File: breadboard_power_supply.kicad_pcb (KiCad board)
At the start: 2 copper layers, 46.7 x 52.3 mm, 18 parts, among them J1 Barrel_Jack_Switch, J2 locked, J3 Conn_01x02_Male, J4 Screw_Terminal_01x02, J5 Conn_01x03_Male, J6 Conn_01x03_Male, J7 Screw_Terminal_01x02, U1 LM7805_TO220, U2 LM317_TO-220

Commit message: PCB complete design of the power supply.
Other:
- board text added: "0,2000 mm / 0,0000 mm"
- board text added: "0,3000 mm"
- board text added: "1,6000 mm"
- board text added: "2"
- board text added: "46,8360 mm x 52,4240 mm"
- board text added: "BOARD CHARACTERISTICS"
- board text added: "Board Thickness:"
- board text added: "Board overall dimensions:"
- board text added: "Castellated pads:"
- board text added: "Copper Finish:"
- board text added: "Copper Layer Count:"
- board text added: "Edge card connectors:"
- board text added: "Impedance Control:"
- board text added: "Min hole diameter:"
- board text added: "Min track/spacing:"
- board text added: "No"
- board text added: "None"
- board text added: "Plated Board Edge:"
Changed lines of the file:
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@@
     (effects (font (size 0.8 0.8) (thickness 0.1)))
+  )
+  (gr_text "Castellated pads: " (at 60.694 77.316) (layer "User.1")
+    (effects (font (size 1.5 1.5) (thickness 0.2)) (justify left top))
+  )
+  (gr_text "Min hole diameter: " (at 127.308286 68.286) (layer "User.1")
+    (effects (font (size 1.5 1.5) (thickness 0.2)) (justify left top))
+  )
+  (gr_text "No" (at 152.151143 77.316) (layer "User.1")
+    (effects (font (size 1.5 1.5) (thickness 0.2)) (justify left top))
+  )
+  (gr_text "Copper Layer Count: " (at 60.694 59.256) (layer "User.1")
+    (effects (font (size 1.5 1.5) (thickness 0.2)) (justify left top))
+  )
+  (gr_text "No" (at 93.251143 81.831) (layer "User.1")
+    (effects (font (size 1.5 1.5) (thickness 0.2)) (justify left top))
+  )
+  (gr_text "" (at 127.308286 63.771) (layer "User.1")
+    (effects (font (size 1.5 1.5) (thickness 0.2)) (justify left top))
+  )
+  (gr_text "No" (at 93.251143 77.316) (layer "User.1")
+    (effects (font (size 1.5 1.5) (thickness 0.2)) (justify left top))
+  )
+  (gr_text "Board overall dimensions: " (at 60.694 63.771) (layer "User.1")
+    (effects (font (size 1.5 1.5) (thickness 0.2)) (justify left top))
+  )
+  (gr_text "Copper Finish: " (at 60.694 72.801) (layer "User.1")
+    (effects (font (size 1.5 1.5) (thickness 0.2)) (justify left top))
+  )
+  (gr_text "Edge card connectors: " (at 60.694 81.831) (layer "User.1")
+    (effects (font (size 1.5 1.5) (thickness 0.2)) (justify left top))
+  )
+  (gr_text "2" (at 93.251143 59.256) (layer "User.1")
+    (effects (font (size 1.5 1.5) (thickness 0.2)) (justify left top))
+  )
+  (gr_text "No" (at 152.151143 72.801) (layer "User.1")
+    (effects (font (size 1.5 1.5) (thickness 0.2)) (justify left top))
+  )
+  (gr_text "1,6000 mm" (at 152.151143 59.256) (layer "User.1")
+    (effects (font (size 1.5 1.5) (thickness 0.2)) (justify left top))
+  )
+  (gr_text "Board Thickness: " (at 127.308286 59.256) (layer "User.1")
+    (effects (font (size 1.5 1.5) (thickness 0.2)) (justify left top))
+  )
+  (gr_text "None" (at 93.251143 72.801) (layer "User.1")
+    (effects (font (size 1.5 1.5) (thickness 0.2)) (justify left top))
+  )
+  (gr_text "Min track/spacing: " (at 60.694 68.286) (layer "User.1")
+    (effects (font (size 1.5 1.5) (thickness 0.2)) (justify left top))
+  )
+  (gr_text "0,2000 mm / 0,0000 mm" (at 93.251143 68.286) (layer "User.1")
+    (effects (font (size 1.5 1.5) (thickness 0.2)) (justify left top))
+  )
+  (gr_text "BOARD CHARACTERISTICS" (at 59.944 53.086) (layer "User.1")
+    (effects (font (size 2 2) (thickness 0.4)) (justify left top))
+  )
+  (gr_text "" (at 152.151143 63.771) (layer "User.1")
+    (effects (font (size 1.5 1.5) (thickness 0.2)) (justify left top))
+  )
+  (gr_text "Impedance Control: " (at 127.308286 72.801) (layer "User.1")
+    (effects (font (size 1.5 1.5) (thickness 0.2)) (justify left top))
+  )
+  (gr_text "0,3000 mm" (at 152.151143 68.286) (layer "User.1")
+    (effects (font (size 1.5 1.5) (thickness 0.2)) (justify left top))
+  )
+  (gr_text "Plated Board Edge: " (at 127.308286 77.316) (layer "User.1")
+    (effects (font (size 1.5 1.5) (thickness 0.2)) (justify left top))
+  )
+  (gr_text "46,8360 mm x 52,4240 mm" (at 93.251143 63.771) (layer "User.1")
+    (effects (font (size 1.5 1.5) (thickness 0.2)) (justify left top))
   )
   (dimension (type aligned) (layer "User.1")
@@
     )
   )
+  (group "group-boardCharacteristics" (id 3579cf2f-29b0-46b6-a07d-483fb5586322)
+    (members
+      044dde97-ee2e-473a-9264-ed4dff1893a5
+      15ea3484-2685-47cb-9e01-ec01c6d477b8
+      18d3014d-7089-41b5-ab03-53cc0a265580
+      232ccf4f-3322-4e62-990b-290e6ff36fcd
+      3f96e159-1f3b-4ee7-a46e-e60d78f2137a
+      406d491e-5b01-46dc-a768-fd0992cdb346
+      4160bbf7-ffff-4c5c-a647-5ee58ddecf06
+      42b61d5b-39d6-462b-b2cc-57656078085f
+      661ca2ba-bce5-4308-99a6-de333a625515
+      662bafcb-dcfb-4471-a8a9-f5c777fdf249
+      6d7ff8c0-8a2a-4636-844f-c7210ff3e6f2
+      720ec55a-7c69-4064-b792-ef3dbba4eab9
+      722636b6-8ff0-452f-9357-23deb317d921
+      7582a530-a952-46c1-b7eb-75006524ba29
+      8ae05d37-86b4-45ea-800f-f1f9fb167857
+      93ac15d8-5f91-4361-acff-be4992b93b51
+      96781640-c07e-4eea-a372-067ded96b703
+      bf8d857b-70bf-41ee-a068-5771461e04e9
+      c6462399-f2e4-4f1a-b34a-b49a04c8bdb9
+      d115a0df-1034-4583-83af-ff1cb8acfa17
+      d4ef5db0-5fba-4fcd-ab64-2ef2646c5c6d
+      e000728f-e3c5-4fc4-86af-db9ceb3a6542
+      f284b1e2-75a4-4a3f-a5f4-6f05f15fb4f5
+    )
+  )

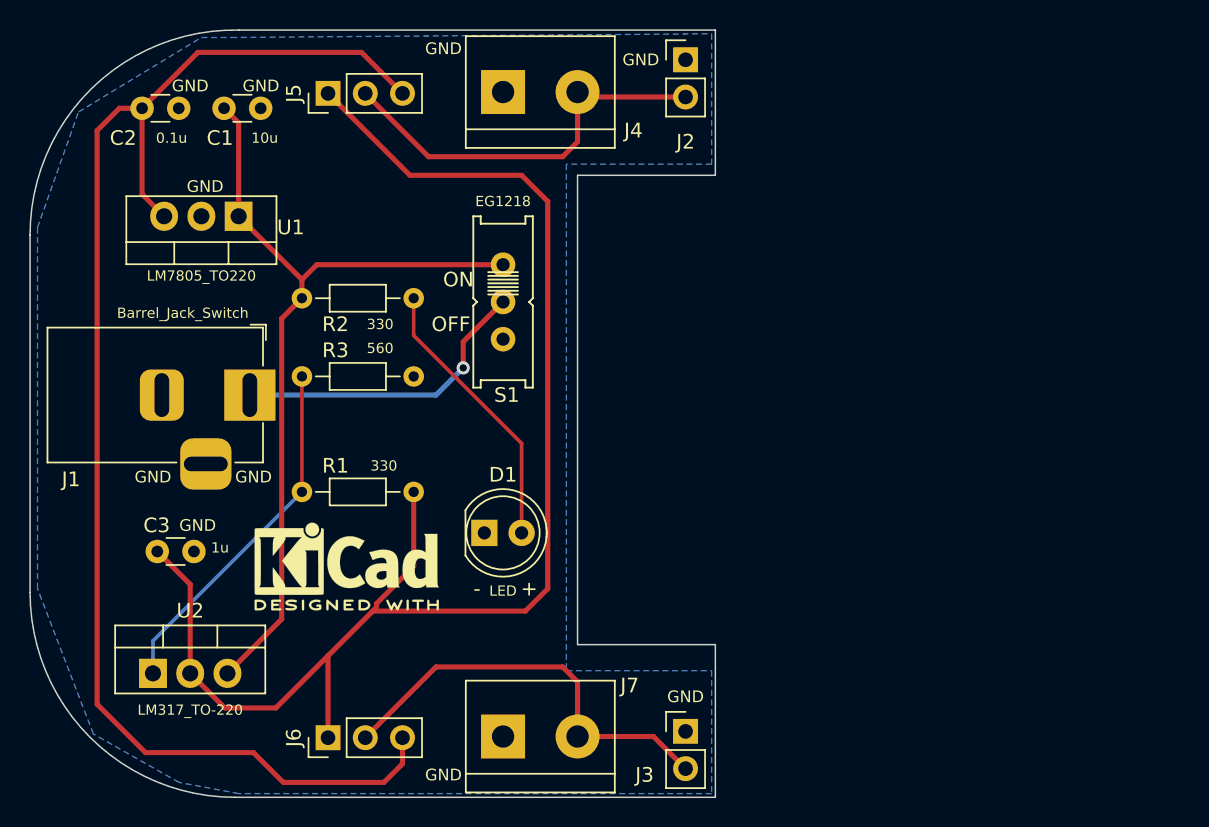
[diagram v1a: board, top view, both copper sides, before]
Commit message: back-up recovery
I lost the old document, and tried to bring it back extracting a backups file from Supply_and_Sensors branch
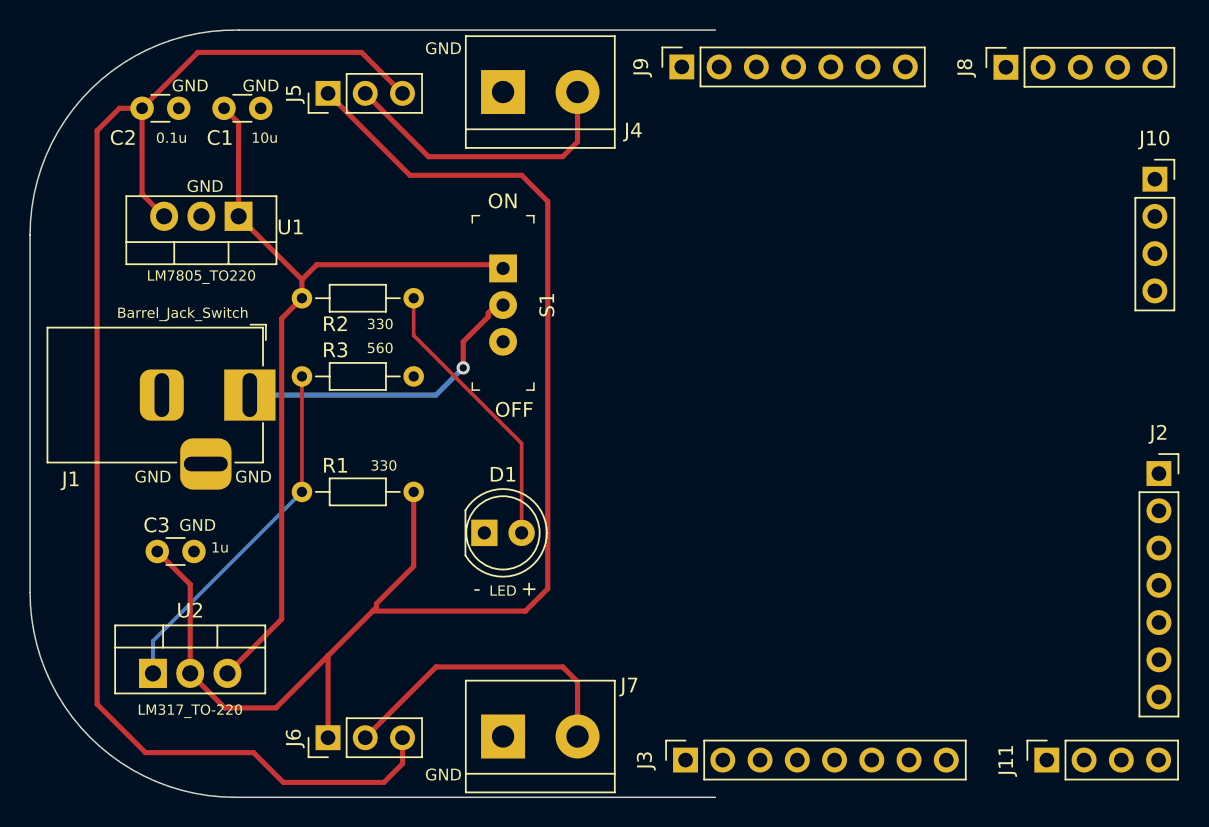
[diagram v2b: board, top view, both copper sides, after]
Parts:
- removed REF**: KiCad-Logo2_5mm_SilkScreen, Symbol:KiCad-Logo2_5mm_SilkScreen
- added J10: Conn_01x04_Male, Connector_PinSocket_2.54mm:PinSocket_1x04_P2.54mm_Vertical, F.Cu at (247.9, 54.9)
- added J11: Conn_01x04_Male, Connector_PinSocket_2.54mm:PinSocket_1x04_P2.54mm_Vertical, F.Cu at (240.5, 94.5)
- added J8: Conn_01x05_Male, Connector_PinSocket_2.54mm:PinSocket_1x05_P2.54mm_Vertical, F.Cu at (237.7, 47.2)
- added J9: Conn_01x07_Male, Connector_PinSocket_2.54mm:PinSocket_1x07_P2.54mm_Vertical, F.Cu at (215.6, 47.2)
- J2: value locked -> Conn_01x07_Male; footprint Connector_PinHeader_2.54mm:PinHeader_1x02_P2.54mm_Vertical -> Connector_PinSocket_2.54mm:PinSocket_1x07_P2.54mm_Vertical
- J3: value Conn_01x02_Male -> Conn_01x08_Male; footprint Connector_PinHeader_2.54mm:PinHeader_1x02_P2.54mm_Vertical -> Connector_PinSocket_2.54mm:PinSocket_1x08_P2.54mm_Vertical
- S1: footprint EG1218:EG1218 -> digkey_slide_switch:Switch_Slide_11.6x4mm_EG1218
- moved J2 42.9 mm to (248.2, 75.0)
- moved S1 2.29 mm to (203.5, 61.0)
- moved J3 1.96 mm to (215.9, 94.5), turned to 90 degrees
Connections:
- J2 pad 1: GND -> /Connectors/5V
- J2 pad 2: /PWR_OUT_TOP -> unconnected-(J2-Pad2)
- J3 pad 1: GND -> /Connectors/5V
- J3 pad 2: /PWR_OUT_BOTTOM -> /Connectors/GND
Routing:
- net /PWR_OUT_BOTTOM: track 28.9 -> 20.6 mm
- net /PWR_OUT_TOP: track 27.6 -> 20.6 mm
- removed copper zone on B.Cu, net GND
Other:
- outline, holes or cut-outs redrawn
- board text removed: "Version 1"

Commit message: Revert "Project Target Description"
This reverts commit 992a993e3ba41f038e621602d57108eb9190e08b.
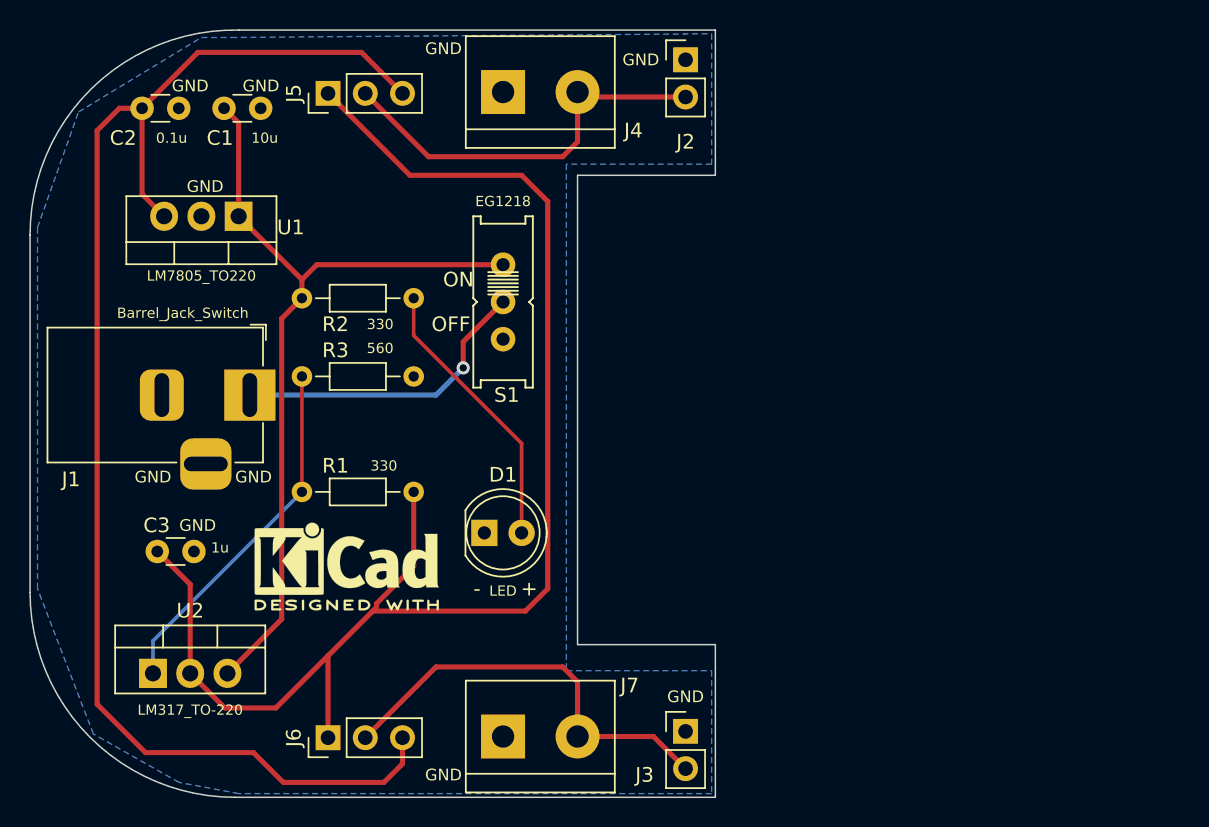
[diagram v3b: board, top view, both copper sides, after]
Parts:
- removed J10, J11: Conn_01x04_Male, Connector_PinSocket_2.54mm:PinSocket_1x04_P2.54mm_Vertical
- removed J8: Conn_01x05_Male, Connector_PinSocket_2.54mm:PinSocket_1x05_P2.54mm_Vertical
- removed J9: Conn_01x07_Male, Connector_PinSocket_2.54mm:PinSocket_1x07_P2.54mm_Vertical
- added REF**: KiCad-Logo2_5mm_SilkScreen, Symbol:KiCad-Logo2_5mm_SilkScreen, F.Cu at (192.8, 81.3)
- J2: value Conn_01x07_Male -> locked; footprint Connector_PinSocket_2.54mm:PinSocket_1x07_P2.54mm_Vertical -> Connector_PinHeader_2.54mm:PinHeader_1x02_P2.54mm_Vertical
- J3: value Conn_01x08_Male -> Conn_01x02_Male; footprint Connector_PinSocket_2.54mm:PinSocket_1x08_P2.54mm_Vertical -> Connector_PinHeader_2.54mm:PinHeader_1x02_P2.54mm_Vertical
- S1: footprint digkey_slide_switch:Switch_Slide_11.6x4mm_EG1218 -> EG1218:EG1218
- moved J2 42.9 mm to (215.9, 46.7)
- moved S1 2.29 mm to (203.5, 63.2)
- moved J3 1.96 mm to (215.9, 92.5), turned to 0 degrees
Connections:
- J2 pad 1: /Connectors/5V -> GND
- J2 pad 2: unconnected-(J2-Pad2) -> /PWR_OUT_TOP
- J3 pad 1: /Connectors/5V -> GND
- J3 pad 2: /Connectors/GND -> /PWR_OUT_BOTTOM
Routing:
- net /PWR_OUT_BOTTOM: track 20.6 -> 28.9 mm
- net /PWR_OUT_TOP: track 20.6 -> 27.6 mm
- added copper zone on B.Cu, net GND
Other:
- outline, holes or cut-outs redrawn
- board text added: "Version 1"
